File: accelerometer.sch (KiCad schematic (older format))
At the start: 5 parts, among them U6 LIS3DH

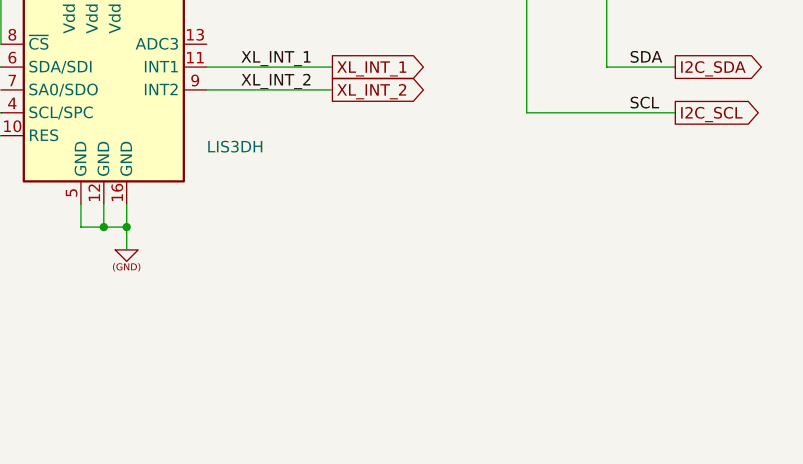
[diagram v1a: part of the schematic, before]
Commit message: accelerometer
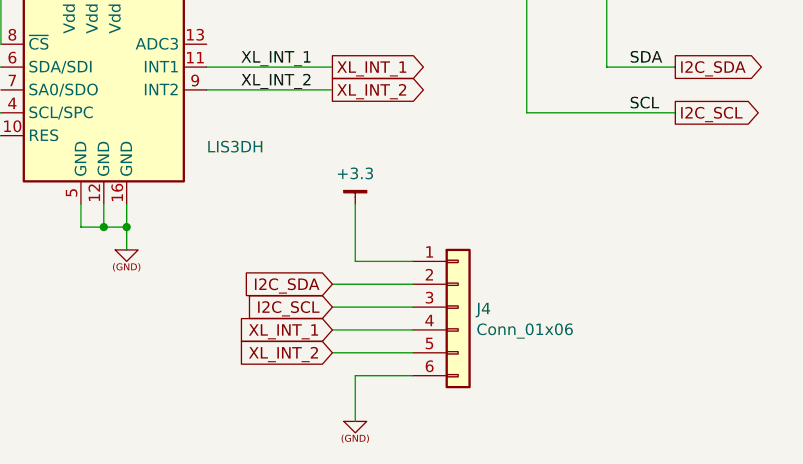
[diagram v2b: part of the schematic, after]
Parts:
- added J4: Conn_01x06, Pin_Headers:Pin_Header_Straight_1x06_Pitch2.54mm, symbol Connector_Generic:Conn_01x06
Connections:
- net (GND): now also J4.6 (Pin_6)
- net +3.3: now also J4.1 (Pin_1)
- net I2C_SCL: now also J4.3 (Pin_3)
- net I2C_SDA: now also J4.2 (Pin_2)
- net XL_INT_1: now also J4.4 (Pin_4)
- net XL_INT_2: now also J4.5 (Pin_5)
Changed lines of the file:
@@
 Text Label 8000 3550 0    50   ~ 0
 SCL
+$Comp
+L Connector_Generic:Conn_01x06 J4
+U 1 1 5D1D81D8
+P 7250 4400
+F 0 "J4" H 7330 4392 50  0000 L CNN
+F 1 "Conn_01x06" H 7330 4301 50  0000 L CNN
+F 2 "Pin_Headers:Pin_Header_Straight_1x06_Pitch2.54mm" H 7250 4400 50  0001 C CNN
+F 3 "~" H 7250 4400 50  0001 C CNN
+	1    7250 4400
+	1    0    0    -1
+$EndComp
+$Comp
+L power:+3.3 #PWR0104
+U 1 1 5D1D8E53
+P 6800 3950
+F 0 "#PWR0104" H 6800 4000 30  0001 C CNN
+F 1 "+3.3" H 6800 4083 50  0000 C CNN
+F 2 "" H 6800 3950 60  0000 C CNN
+F 3 "" H 6800 3950 60  0000 C CNN
+	1    6800 3950
+	1    0    0    -1
+$EndComp
+$Comp
+L power:(GND) #PWR0105
+U 1 1 5D1D97A2
+P 6800 4900
+F 0 "#PWR0105" H 6800 4900 30  0001 C CNN
+F 1 "(GND)" H 6800 4900 30  0001 C CNN
+F 2 "" H 6800 4900 60  0000 C CNN
+F 3 "" H 6800 4900 60  0000 C CNN
+	1    6800 4900
+	1    0    0    -1
+$EndComp
+Wire Wire Line
+	7050 4200 6800 4200
+Wire Wire Line
+	6800 4200 6800 3950
+Wire Wire Line
+	7050 4700 6800 4700
+Wire Wire Line
+	6800 4700 6800 4900
+Text GLabel 6700 4300 0    50   Input ~ 0
+I2C_SDA
+Text GLabel 6700 4400 0    50   Input ~ 0
+I2C_SCL
+Text GLabel 6700 4500 0    50   Input ~ 0
+XL_INT_1
+Text GLabel 6700 4600 0    50   Input ~ 0
+XL_INT_2
+Wire Wire Line
+	6700 4300 7050 4300
+Wire Wire Line
+	6700 4400 7050 4400
+Wire Wire Line
+	6700 4500 7050 4500
+Wire Wire Line
+	6700 4600 7050 4600
 $EndSCHEMATC

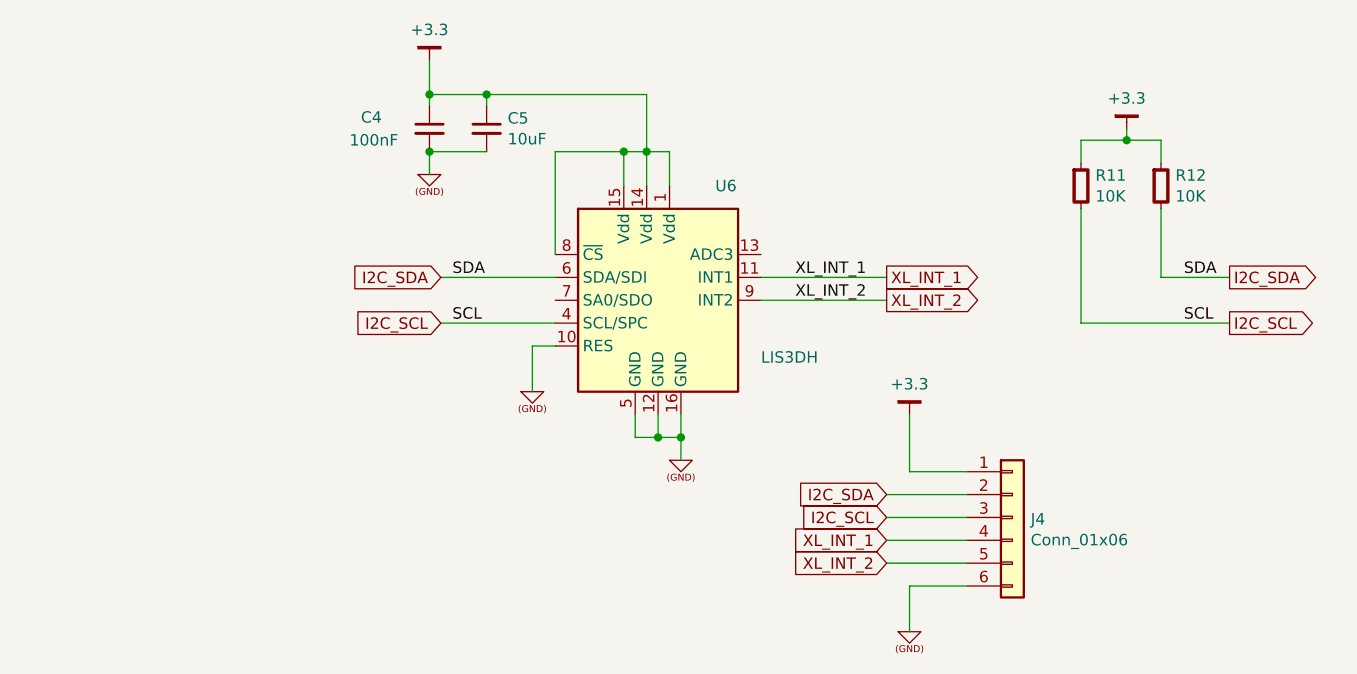
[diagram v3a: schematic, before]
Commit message: Initial
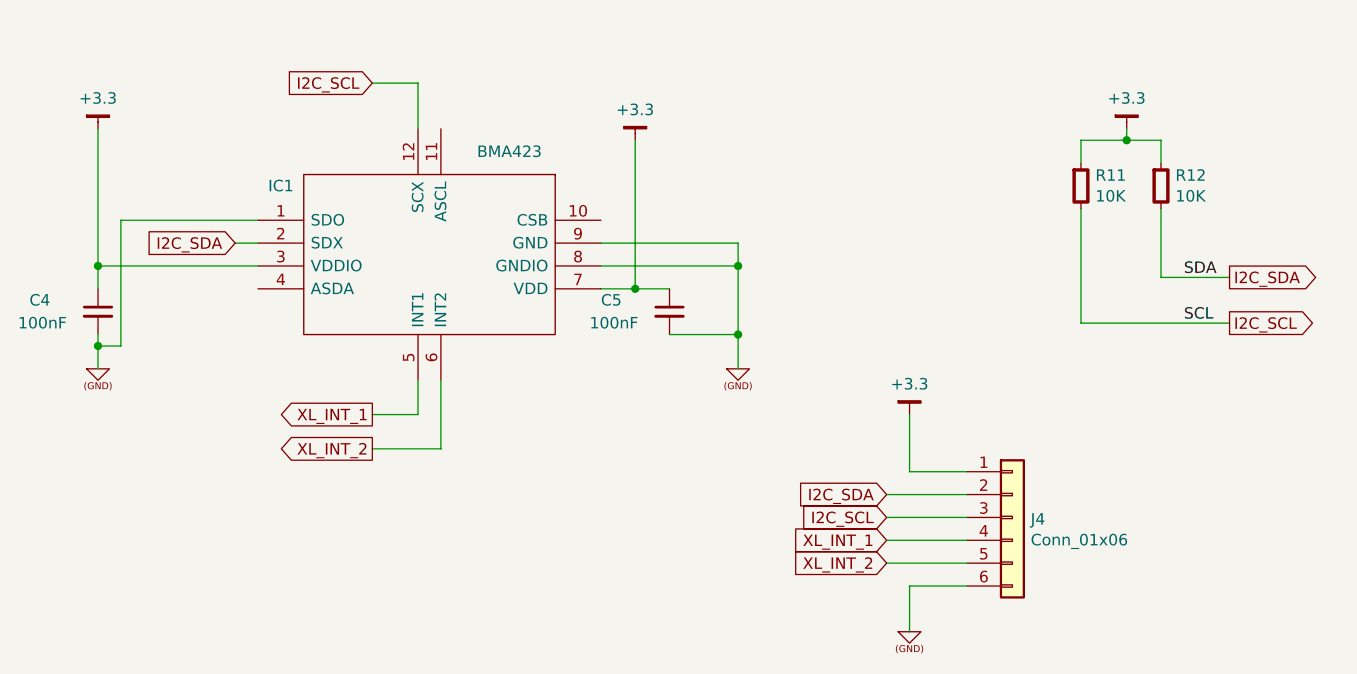
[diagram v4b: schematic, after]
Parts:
- removed U6: LIS3DH, my-fp-library:LGA-16_3x3mm, symbol accel:LIS3DH
- added IC1: BMA423, SamacSys_Parts:BMA423, symbol SamacSys_Parts:BMA423
- C4: footprint Capacitors_SMD:C_0805 -> Capacitors_SMD:C_0603_HandSoldering
- C5: value 10uF -> 100nF; footprint Capacitors_SMD:C_0805 -> Capacitors_SMD:C_0603_HandSoldering
- R11, R12: footprint Resistors_SMD:R_0805 -> Resistors_SMD:R_0603_HandSoldering
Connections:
- net (GND): now also IC1.1 (SDO), IC1.8 (GNDIO), IC1.9 (GND)
- net +3.3: now also IC1.3 (VDDIO), IC1.7 (VDD)
- net I2C_SCL: now also IC1.12 (SCX)
- net I2C_SDA: now also IC1.2 (SDX)
- net XL_INT_1: now also IC1.5 (INT1)
- net XL_INT_2: now also IC1.6 (INT2)
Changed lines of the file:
@@
 $Descr A4 11693 8268
 encoding utf-8
-Sheet 4 5
+Sheet 3 3
 Title ""
 Date ""
@@
 $EndDescr
 $Comp
-L accel:LIS3DH U6
-U 1 1 5D09FBC0
-P 5650 3450
-F 0 "U6" H 5950 3950 50  0000 L CNN
-F 1 "LIS3DH" H 6150 3200 50  0000 L CNN
-F 2 "my-fp-library:LGA-16_3x3mm" H 5650 2850 50  0001 C CNN
-F 3 "http://www.st.com/st-web-ui/static/active/en/resource/technical/document/datasheet/CD00250937.pdf" H 5550 3700 50  0001 C CNN
-	1    5650 3450
-	1    0    0    -1
-$EndComp
-$Comp
-L power:(GND) #PWR0118
-U 1 1 5D09FE5A
-P 5800 4150
-F 0 "#PWR0118" H 5800 4150 30  0001 C CNN
-F 1 "(GND)" H 5800 4150 30  0001 C CNN
-F 2 "" H 5800 4150 60  0000 C CNN
-F 3 "" H 5800 4150 60  0000 C CNN
-	1    5800 4150
-	1    0    0    -1
-$EndComp
-Wire Wire Line
-	5800 3950 5800 4050
-Wire Wire Line
-	5700 3950 5700 4050
-Wire Wire Line
-	5700 4050 5800 4050
-Connection ~ 5800 4050
-Wire Wire Line
-	5800 4050 5800 4150
-Wire Wire Line
-	5600 3950 5600 4050
-Wire Wire Line
-	5600 4050 5700 4050
-Connection ~ 5700 4050
-$Comp
-L power:(GND) #PWR0119
-U 1 1 5D0A007A
-P 5150 3850
-F 0 "#PWR0119" H 5150 3850 30  0001 C CNN
-F 1 "(GND)" H 5150 3850 30  0001 C CNN
-F 2 "" H 5150 3850 60  0000 C CNN
-F 3 "" H 5150 3850 60  0000 C CNN
-	1    5150 3850
-	1    0    0    -1
-$EndComp
-Wire Wire Line
-	5250 3650 5150 3650
-Wire Wire Line
-	5150 3650 5150 3850
-Wire Wire Line
-	5250 3550 4750 3550
-Wire Wire Line
-	5250 3350 4750 3350
-Text Label 4800 3350 0    50   ~ 0
-SDA
-Text Label 4800 3550 0    50   ~ 0
-SCL
-Text GLabel 4750 3350 0    50   Input ~ 0
-I2C_SDA
-Text GLabel 4750 3550 0    50   Input ~ 0
-I2C_SCL
-Wire Wire Line
-	6150 3450 6700 3450
-Wire Wire Line
-	6150 3350 6700 3350
-Text Label 6300 3350 0    50   ~ 0
-XL_INT_1
-Text Label 6300 3450 0    50   ~ 0
-XL_INT_2
-Text GLabel 6700 3350 2    50   Output ~ 0
-XL_INT_1
-Text GLabel 6700 3450 2    50   Output ~ 0
-XL_INT_2
-$Comp
-L power:+3.3 #PWR0120
-U 1 1 5D0A0ABC
-P 4700 2400
-F 0 "#PWR0120" H 4700 2450 30  0001 C CNN
-F 1 "+3.3" H 4700 2533 50  0000 C CNN
-F 2 "" H 4700 2400 60  0000 C CNN
-F 3 "" H 4700 2400 60  0000 C CNN
-	1    4700 2400
-	1    0    0    -1
-$EndComp
-Wire Wire Line
-	5750 2950 5750 2800
-Wire Wire Line
-	5750 2800 5650 2800
-Wire Wire Line
-	5650 2950 5650 2800
-Connection ~ 5650 2800
-Wire Wire Line
-	5650 2800 5550 2800
-Wire Wire Line
-	5550 2950 5550 2800
-$Comp
-L power:(GND) #PWR0121
-U 1 1 5D0A13E6
-P 4700 2900
-F 0 "#PWR0121" H 4700 2900 30  0001 C CNN
-F 1 "(GND)" H 4700 2900 30  0001 C CNN
-F 2 "" H 4700 2900 60  0000 C CNN
-F 3 "" H 4700 2900 60  0000 C CNN
-	1    4700 2900
-	1    0    0    -1
-$EndComp
-$Comp
-L Device:C_Small C5
-U 1 1 5D0A1A79
-P 4950 2700
-F 0 "C5" H 5042 2746 50  0000 L CNN
-F 1 "10uF" H 5042 2655 50  0000 L CNN
-F 2 "Capacitors_SMD:C_0805" H 4950 2700 50  0001 C CNN
-F 3 "~" H 4950 2700 50  0001 C CNN
-	1    4950 2700
-	1    0    0    -1
-$EndComp
-$Comp
-L Device:C_Small C4
-U 1 1 5D0A1B09
-P 4700 2700
-F 0 "C4" H 4400 2750 50  0000 L CNN
-F 1 "100nF" H 4350 2650 50  0000 L CNN
-F 2 "Capacitors_SMD:C_0805" H 4700 2700 50  0001 C CNN
-F 3 "~" H 4700 2700 50  0001 C CNN
-	1    4700 2700
-	1    0    0    -1
-$EndComp
-Wire Wire Line
-	4950 2550 4950 2600
-Wire Wire Line
-	4950 2800 4700 2800
-Wire Wire Line
-	4700 2800 4700 2900
-Connection ~ 4700 2800
-Wire Wire Line
-	4700 2600 4700 2550
-Wire Wire Line
-	4950 2550 4700 2550
-Connection ~ 4950 2550
-Connection ~ 4700 2550
-Wire Wire Line
-	4700 2550 4700 2400
-Wire Wire Line
-	5650 2550 5650 2800
-Wire Wire Line
-	4950 2550 5650 2550
-Wire Wire Line
-	5250 3250 5250 2800
-Wire Wire Line
-	5250 2800 5550 2800
-Connection ~ 5550 2800
-$Comp
 L power:+3.3 #PWR0122
 U 1 1 5D0B441E
@@
 F 0 "R11" H 7613 2996 50  0000 L CNN
 F 1 "10K" H 7613 2905 50  0000 L CNN
-F 2 "Resistors_SMD:R_0805" H 7550 3000 60  0001 C CNN
+F 2 "Resistors_SMD:R_0603_HandSoldering" H 7550 3000 60  0001 C CNN
 F 3 "" H 7550 3000 60  0000 C CNN
 	1    7550 2950
@@
 F 0 "R12" H 7963 2996 50  0000 L CNN
 F 1 "10K" H 7963 2905 50  0000 L CNN
-F 2 "Resistors_SMD:R_0805" H 7900 3000 60  0001 C CNN
+F 2 "Resistors_SMD:R_0603_HandSoldering" H 7900 3000 60  0001 C CNN
 F 3 "" H 7900 3000 60  0000 C CNN
 	1    7900 2950
@@
 Wire Wire Line
 	6700 4600 7050 4600
+$Comp
+L SamacSys_Parts:BMA423 IC1
+U 1 1 5EAF31CD
+P 4750 2700
+F 0 "IC1" V 5000 2000 50  0000 C CNN
+F 1 "BMA423" V 4850 3000 50  0000 C CNN
+F 2 "SamacSys_Parts:BMA423" H 5700 3200 50  0001 L CNN
+F 3 "https://componentsearchengine.com/Datasheets/1/BMA423.pdf" H 5700 3100 50  0001 L CNN
+F 4 "Accelerometers Triaxial low-g 12bit Acceleration Sensor" H 5700 3000 50  0001 L CNN "Description"
+F 5 "1" H 5700 2900 50  0001 L CNN "Height"
+F 6 "262-BMA423" H 5700 2800 50  0001 L CNN "Mouser Part Number"
+F 7 "https://www.mouser.com/Search/Refine.aspx?Keyword=262-BMA423" H 5700 2700 50  0001 L CNN "Mouser Price/Stock"
+F 8 "Bosch Sensortec" H 5700 2600 50  0001 L CNN "Manufacturer_Name"
+F 9 "BMA423" H 5700 2500 50  0001 L CNN "Manufacturer_Part_Number"
+	1    4750 2700
+	0    1    1    0
+$EndComp
+$Comp
+L power:(GND) #PWR07
+U 1 1 5EAF52DD
+P 6050 3750
+F 0 "#PWR07" H 6050 3750 30  0001 C CNN
+F 1 "(GND)" H 6050 3750 30  0001 C CNN
+F 2 "" H 6050 3750 60  0000 C CNN
+F 3 "" H 6050 3750 60  0000 C CNN
+	1    6050 3750
+	1    0    0    -1
+$EndComp
+Wire Wire Line
+	5450 3200 6050 3200
+Wire Wire Line
+	6050 3200 6050 3300
+Wire Wire Line
+	5450 3300 6050 3300
+Connection ~ 6050 3300
+Wire Wire Line
+	6050 3300 6050 3600
+$Comp
+L power:+3.3 #PWR06
+U 1 1 5EAF7E3F
+P 5600 2750
+F 0 "#PWR06" H 5600 2800 30  0001 C CNN
+F 1 "+3.3" H 5600 2883 50  0000 C CNN
+F 2 "" H 5600 2750 60  0000 C CNN
+F 3 "" H 5600 2750 60  0000 C CNN
+	1    5600 2750
+	1    0    0    -1
+$EndComp
+Wire Wire Line
+	5450 3400 5600 3400
+Wire Wire Line
+	5600 3400 5600 2750
+$Comp
+L Device:C_Small C5
+U 1 1 5EAFA5CD
+P 5750 3500
+F 0 "C5" H 5450 3550 50  0000 L CNN
+F 1 "100nF" H 5400 3450 50  0000 L CNN
+F 2 "Capacitors_SMD:C_0603_HandSoldering" H 5750 3500 50  0001 C CNN
+F 3 "~" H 5750 3500 50  0001 C CNN
+	1    5750 3500
+	1    0    0    -1
+$EndComp
+Wire Wire Line
+	5600 3400 5750 3400
+Connection ~ 5600 3400
+Wire Wire Line
+	5750 3600 6050 3600
+Connection ~ 6050 3600
+Wire Wire Line
+	6050 3600 6050 3750
+$Comp
+L power:+3.3 #PWR04
+U 1 1 5EAFDBA1
+P 3250 2700
+F 0 "#PWR04" H 3250 2750 30  0001 C CNN
+F 1 "+3.3" H 3250 2833 50  0000 C CNN
+F 2 "" H 3250 2700 60  0000 C CNN
+F 3 "" H 3250 2700 60  0000 C CNN
+	1    3250 2700
+	1    0    0    -1
+$EndComp
+Wire Wire Line
+	3250 3300 3250 2700
+$Comp
+L power:(GND) #PWR05
+U 1 1 5EAFEFC5
+P 3250 3750
+F 0 "#PWR05" H 3250 3750 30  0001 C CNN
+F 1 "(GND)" H 3250 3750 30  0001 C CNN
+F 2 "" H 3250 3750 60  0000 C CNN
+F 3 "" H 3250 3750 60  0000 C CNN
+	1    3250 3750
+	1    0    0    -1
+$EndComp
+$Comp
+L Device:C_Small C4
+U 1 1 5EAFF675
+P 3250 3500
+F 0 "C4" H 2950 3550 50  0000 L CNN
+F 1 "100nF" H 2900 3450 50  0000 L CNN
+F 2 "Capacitors_SMD:C_0603_HandSoldering" H 3250 3500 50  0001 C CNN
+F 3 "~" H 3250 3500 50  0001 C CNN
+	1    3250 3500
+	1    0    0    -1
+$EndComp
+Wire Wire Line
+	3250 3300 3250 3400
+Connection ~ 3250 3300
+Wire Wire Line
+	3250 3600 3250 3650
+Text GLabel 4450 2500 0    50   Input ~ 0
+I2C_SCL
+Wire Wire Line
+	4450 2500 4650 2500
+Wire Wire Line
+	4650 2500 4650 2700
+Text GLabel 4450 3950 0    50   Output ~ 0
+XL_INT_1
+Text GLabel 4450 4100 0    50   Output ~ 0
+XL_INT_2
+Wire Wire Line
+	4650 3800 4650 3950
+Wire Wire Line
+	4650 3950 4450 3950
+Wire Wire Line
+	4750 3800 4750 4100
+Wire Wire Line
+	4750 4100 4450 4100
+Text GLabel 3850 3200 0    50   Input ~ 0
+I2C_SDA
+Wire Wire Line
+	3350 3100 3350 3650
+Wire Wire Line
+	3350 3650 3250 3650
+Connection ~ 3250 3650
+Wire Wire Line
+	3250 3650 3250 3750
+Wire Wire Line
+	3850 3200 3950 3200
+Wire Wire Line
+	3350 3100 3950 3100
+Wire Wire Line
+	3250 3300 3950 3300
 $EndSCHEMATC
